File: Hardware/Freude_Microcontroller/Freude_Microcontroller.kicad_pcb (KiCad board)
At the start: 4 copper layers, 20.3 x 21.7 mm, 22 parts, among them J2 Conn_01x05_Female, J3 Conn_01x06_Female, J4 Conn_01x06_Female, SW1 B3FS-1015P`, U2 STM32L432KBUx, Y1 Crystal_GND24

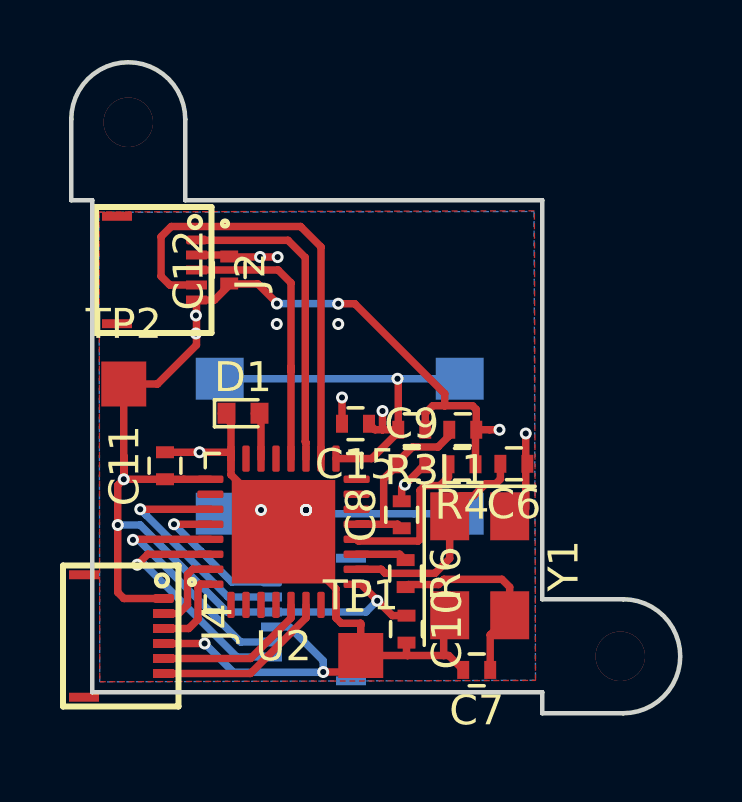
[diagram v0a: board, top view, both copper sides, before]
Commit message: silk layout, proto release candidate
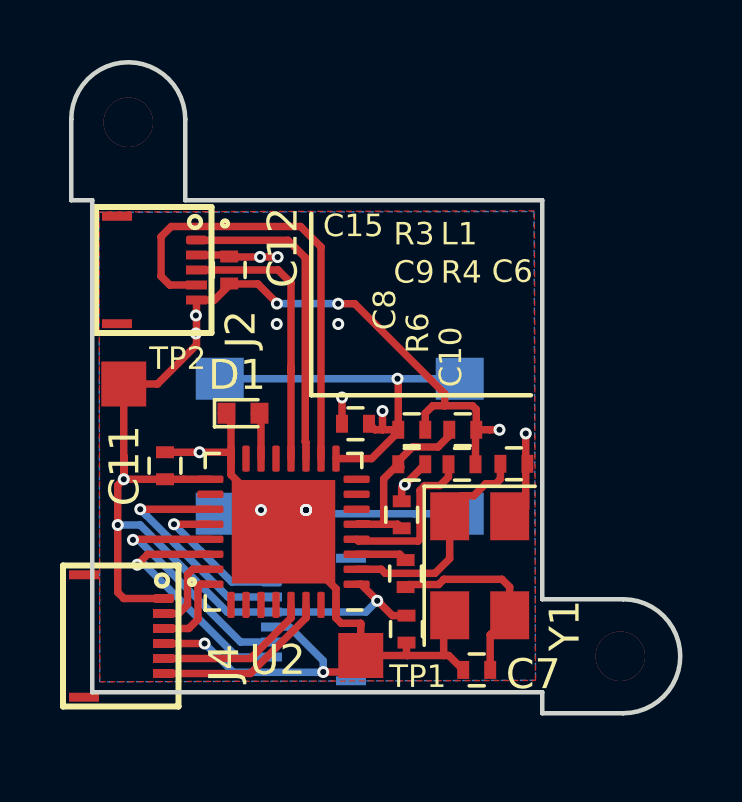
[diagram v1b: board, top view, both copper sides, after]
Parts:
- renumbered REF** to Outline
